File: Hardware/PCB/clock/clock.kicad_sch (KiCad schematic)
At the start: 51 parts, among them J1 Synth_power_2x5, J2 AudioJack2, J3 AudioJack2, J4 AudioJack2, J5 AudioJack2, J6 AudioJack2, J7 AudioJack2, Q1 2N3904, SW1 RotaryEncoder, SW2 SW_Push, U1 40106

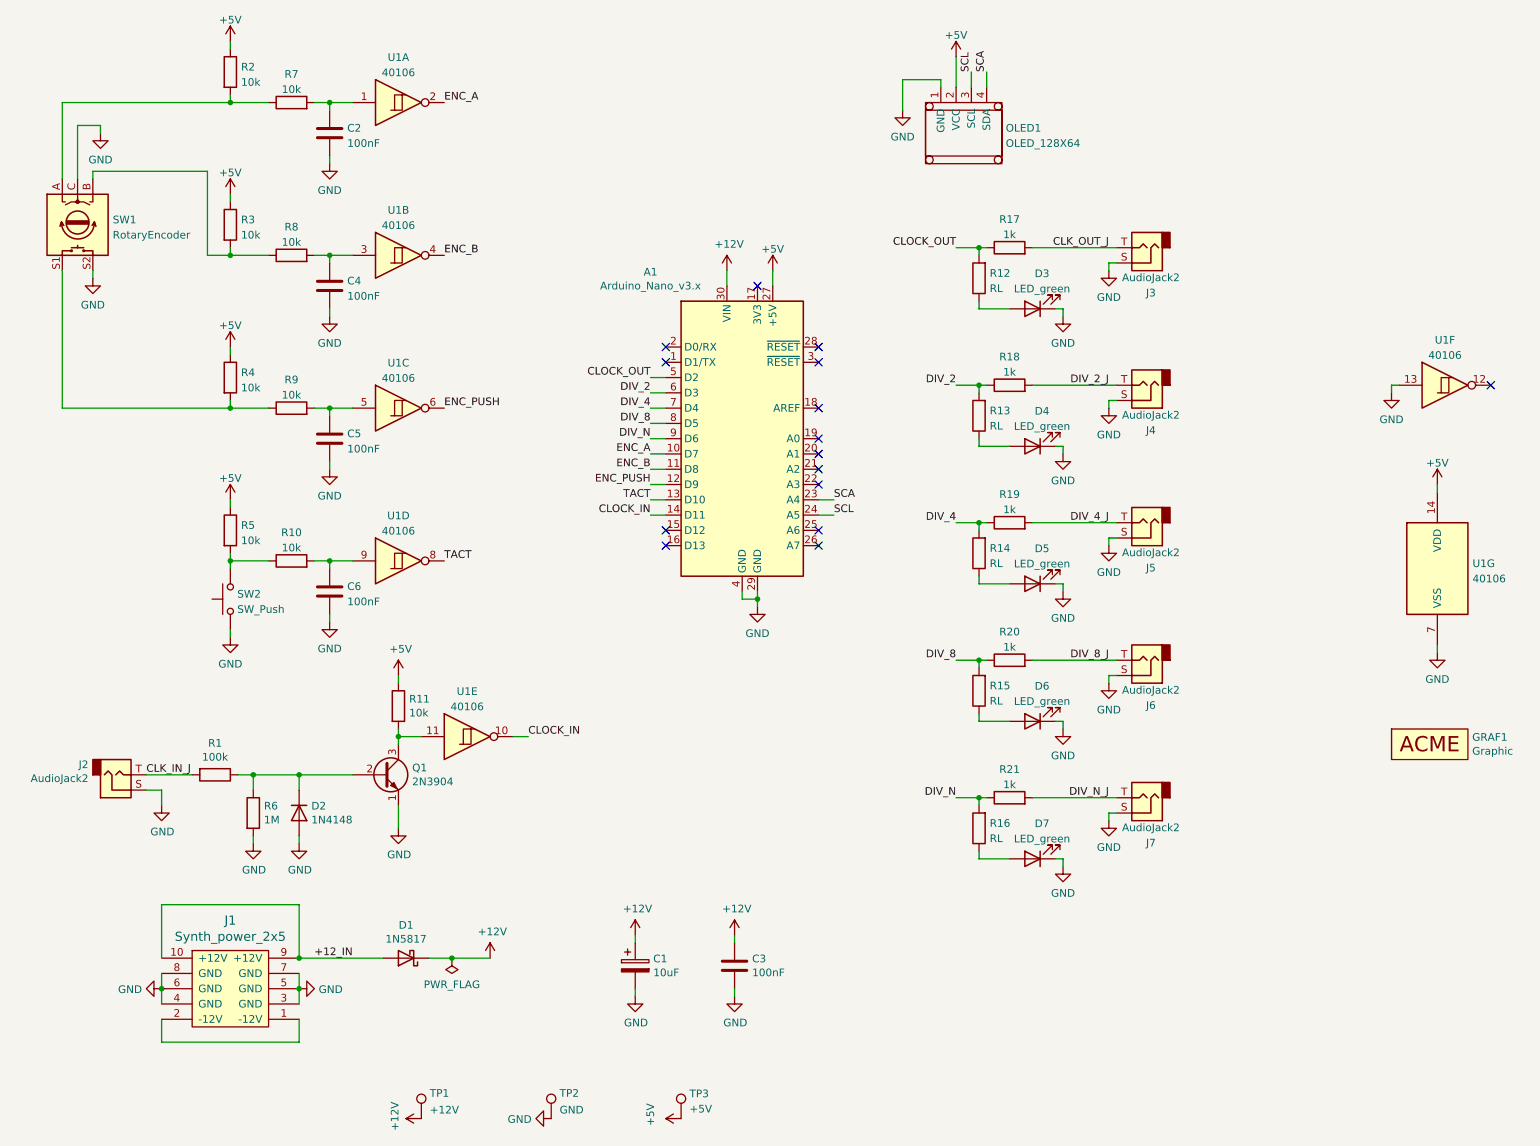
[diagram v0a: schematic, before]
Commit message: Initial layout, README update, software cleanup
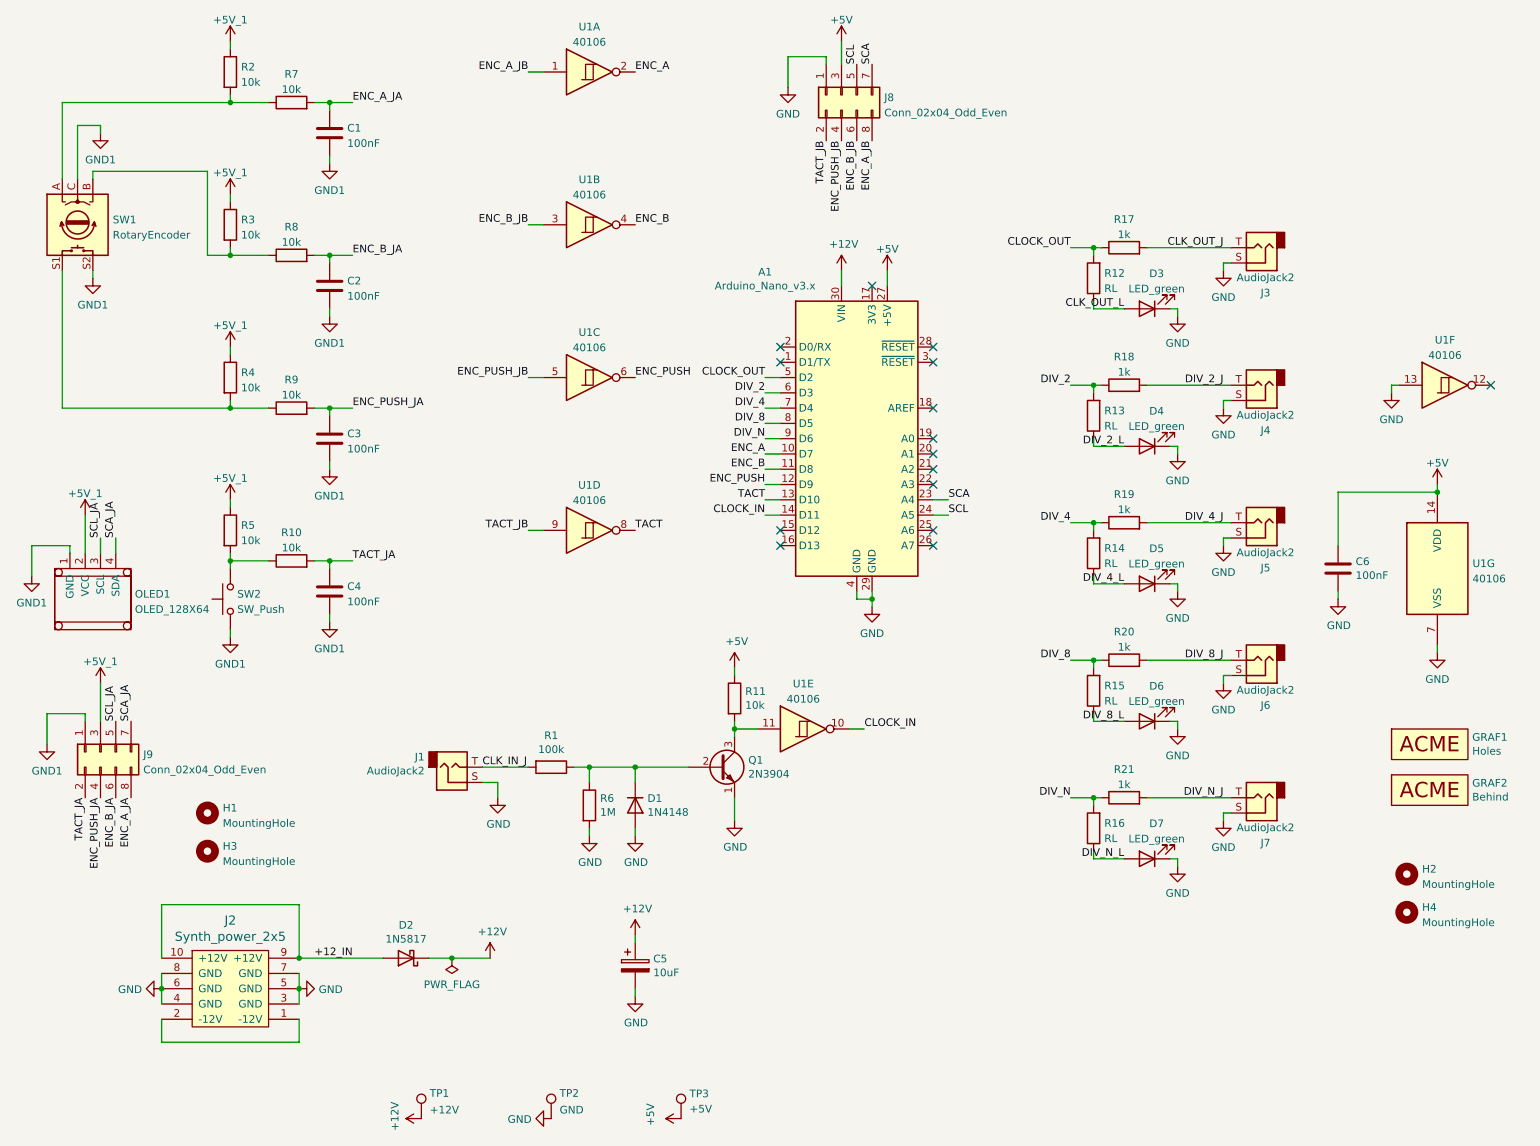
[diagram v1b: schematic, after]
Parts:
- added GRAF2: Behind, clock:clock_panel_behind, symbol ao_symbols:Graphic
- added H1, H2, H3, H4: MountingHole, ao_tht:MountingHole_3.2mm_M3, symbol ao_symbols:MountingHole
- added J8, J9: Conn_02x04_Odd_Even, Connector_IDC:IDC-Header_2x04_P2.54mm_Vertical, symbol Connector_Generic:Conn_02x04_Odd_Even
- D3, D4, D5, D6, D7: footprint (none) -> ao_tht:LED_D5.0mm
- GRAF1: value Graphic -> Holes; footprint clock:clock_panel_mockup -> clock:clock_panel_holes
- OLED1: footprint (none) -> Connector_PinHeader_2.54mm:PinHeader_1x04_P2.54mm_Vertical
- R1, R10, R11, R12, R13, R14, R15, R16, R17, R18, R19, R2, R20, R21, R3, R4, R5, R6, R7, R8, R9: footprint ao_tht:R_Axial_DIN0207_L6.3mm_D2.5mm_P10.16mm_Horizontal -> ao_tht:R_Axial_DIN0204_L3.6mm_D1.6mm_P7.62mm_Horizontal
- SW1: footprint (none) -> ao_tht:RotaryEncoder_Bourns-PEC11R-4xxxF-Sxxxx-Switch_Vertical_H20mm
- SW2: footprint (none) -> ao_tht:Tactile_E-switch_TL1100F160Q
- U1: footprint (none) -> ao_tht:DIP-14_W7.62mm_Socket_LongPads
- renumbered C2 to C1, C4 to C2, C5 to C3, C6 to C4, C1 to C5, C3 to C6, D2 to D1, D1 to D2, J2 to J1, J1 to J2
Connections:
- net +12V: no longer C6.1
- net +5V: now also C6.1, J8.3 (Pin_3); no longer OLED1.2 (VCC), R2.1, R3.1, R4.1, R5.1
- net GND: now also J8.1 (Pin_1); no longer C1.2, C2.2, C3.2, C4.2, OLED1.1 (GND), SW1.C, SW1.S2, SW2.1
- net SCA: now also J8.7 (Pin_7); no longer OLED1.4 (SDA)
- net SCL: now also J8.5 (Pin_5); no longer OLED1.3 (SCL)
- net ENC_A_JA: now reaches C1.1, R7.2
- net ENC_A_JA: now also J9.8 (Pin_8); no longer U1.1
- net TACT_JA: now reaches C4.1, R10.2
- net TACT_JA: now also J9.2 (Pin_2); no longer U1.9
- net ENC_B_JA: now reaches C2.1, R8.2
- net ENC_B_JA: now also J9.6 (Pin_6); no longer U1.3
- net CLK_OUT_L: now reaches D3.2 (A), R12.1
- net DIV_2_L: now reaches D4.2 (A), R13.1
- net DIV_8_L: now reaches D6.2 (A), R15.1
- net ENC_PUSH_JA: now reaches C3.1, R9.2
- net ENC_PUSH_JA: now also J9.4 (Pin_4); no longer U1.5
- net DIV_4_L: now reaches D5.2 (A), R14.1
- net DIV_N_L: now reaches D7.2 (A), R16.1
- new net +5V_1: J9.3 (Pin_3), OLED1.2 (VCC), R2.1, R3.1, R4.1, R5.1
- new net ENC_A_JB: J8.8 (Pin_8), U1.1
- new net ENC_B_JB: J8.6 (Pin_6), U1.3
- new net ENC_PUSH_JB: J8.4 (Pin_4), U1.5
- new net GND1: C1.2, C2.2, C3.2, C4.2, J9.1 (Pin_1), OLED1.1 (GND), SW1.C, SW1.S2, SW2.1
- new net SCA_JA: J9.7 (Pin_7), OLED1.4 (SDA)
- new net SCL_JA: J9.5 (Pin_5), OLED1.3 (SCL)
- new net TACT_JB: J8.2 (Pin_2), U1.9
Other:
- moved on the sheet: A1, C6, D1, D3, D4, D5, D6, D7, J1, J3, J4, J5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

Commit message: Layout revisions
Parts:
- GRAF2: footprint clock:clock_panel_behind -> clock:clock_panel_holes
- OLED1: footprint Connector_PinHeader_2.54mm:PinHeader_1x04_P2.54mm_Vertical -> ao_tht:OLED_MC130GX
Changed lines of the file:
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@@
       (effects (font (size 1.27 1.27)) (justify left))
     )
-    (property "Footprint" "clock:clock_panel_behind" (id 2) (at 250.19 144.78 0)
+    (property "Footprint" "clock:clock_panel_holes" (id 2) (at 250.19 144.78 0)
       (effects (font (size 1.27 1.27)) hide)
     )
@@
       (effects (font (size 1.27 1.27)) (justify left))
     )
-    (property "Footprint" "Connector_PinHeader_2.54mm:PinHeader_1x04_P2.54mm_Vertical" (id 2) (at 27.94 113.03 0)
+    (property "Footprint" "ao_tht:OLED_MC130GX" (id 2) (at 27.94 113.03 0)
       (effects (font (size 1.27 1.27)) hide)
     )
@@
     )
     (path "/3148a9e6-1e75-4e2a-b943-102cc5541cb8"
-      (reference "GRAF2") (unit 1) (value "Behind") (footprint "clock:clock_panel_behind")
+      (reference "GRAF2") (unit 1) (value "Behind") (footprint "clock:clock_panel_holes")
     )
     (path "/9aa227a4-5918-4955-a2f5-b1e4c4fe38eb"
@@
     )
     (path "/33f39dd2-4a83-487c-ae50-5387dc326ac4"
-      (reference "OLED1") (unit 1) (value "OLED_128X64") (footprint "Connector_PinHeader_2.54mm:PinHeader_1x04_P2.54mm_Vertical")
+      (reference "OLED1") (unit 1) (value "OLED_128X64") (footprint "ao_tht:OLED_MC130GX")
     )
     (path "/cc4603d6-fbbe-4d4f-8c75-cc951d37e1ff"
